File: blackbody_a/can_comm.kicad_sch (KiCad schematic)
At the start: 6 parts, among them U3 ISO1044BD

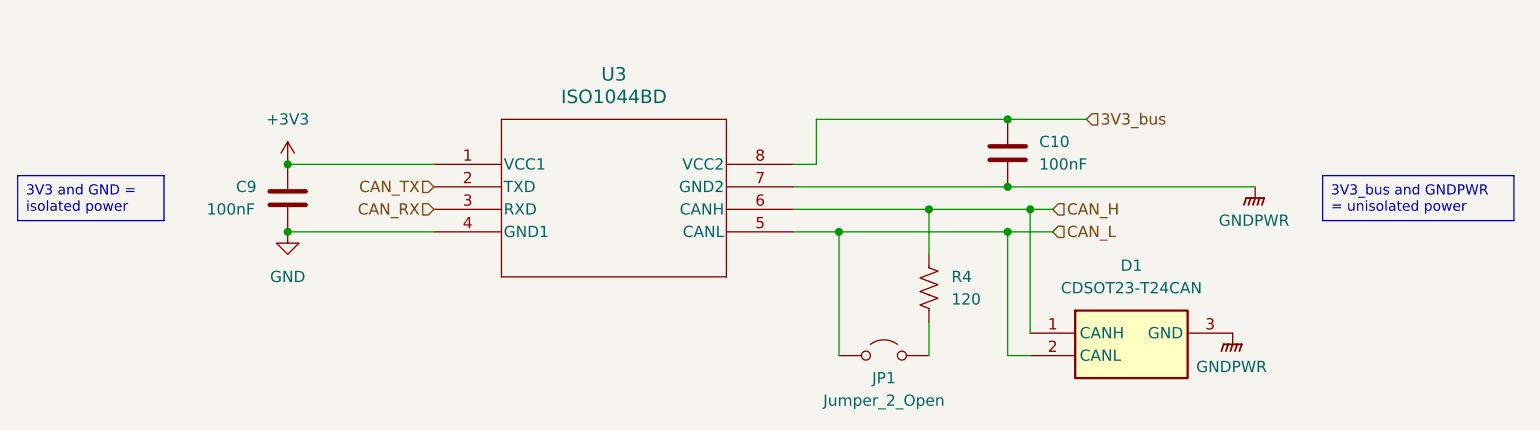
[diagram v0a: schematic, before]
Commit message: Fixed pins, minor changes, removed power isolation
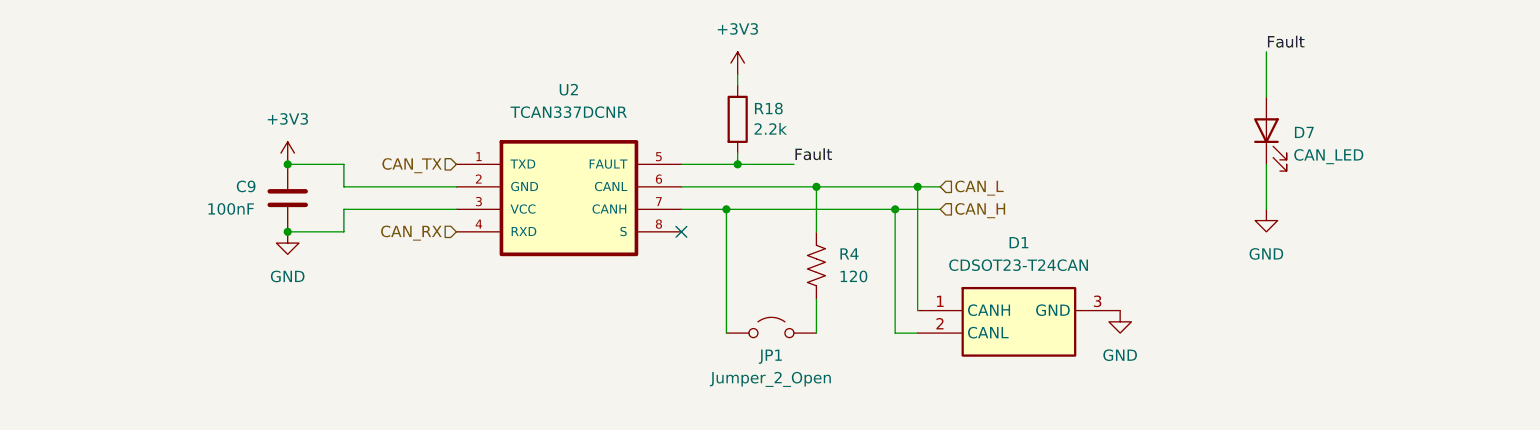
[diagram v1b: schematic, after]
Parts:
- removed C10: 100nF, symbol Device:C
- removed U3: ISO1044BD, SOIC8_D_TEX, symbol ISO1044:ISO1044BD
- added D7: CAN_LED, LED_SMD:LED_0805_2012Metric, symbol Device:LED
- added R18: 2.2k, Resistor_SMD:R_0805_2012Metric, symbol Device:R
- added U2: TCAN337DCNR, TCAN337DCNR:SOT65P280X145-8N, symbol TCAN337DCNR:TCAN337DCNR
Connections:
- net GNDPWR is gone; now on net GND: D1.3 (GND)
- net +3V3: now also R18.1, U2.2 (GND)
- net CAN_H: now also D1.2 (CANL), JP1.1 (A), U2.7 (CANH); no longer D1.1 (CANH), R4.1
- net CAN_L: now also D1.1 (CANH), R4.1, U2.6 (CANL); no longer D1.2 (CANL), JP1.1 (A)
- net CAN_RX: now also U2.4 (RXD)
- net CAN_TX: now also U2.1 (TXD)
- net GND: now also D7.1 (K), U2.3 (VCC)
- new net Fault: D7.2 (A), R18.2, U2.5 (FAULT)
- no-connect marks 0 -> 1
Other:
- moved on the sheet: D1, JP1, R4
